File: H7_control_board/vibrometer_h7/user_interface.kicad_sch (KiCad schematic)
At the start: 21 parts, among them J501 Conn_02x12_Counter_Clockwise, SW501 SW_Push, SW502 SW_Push

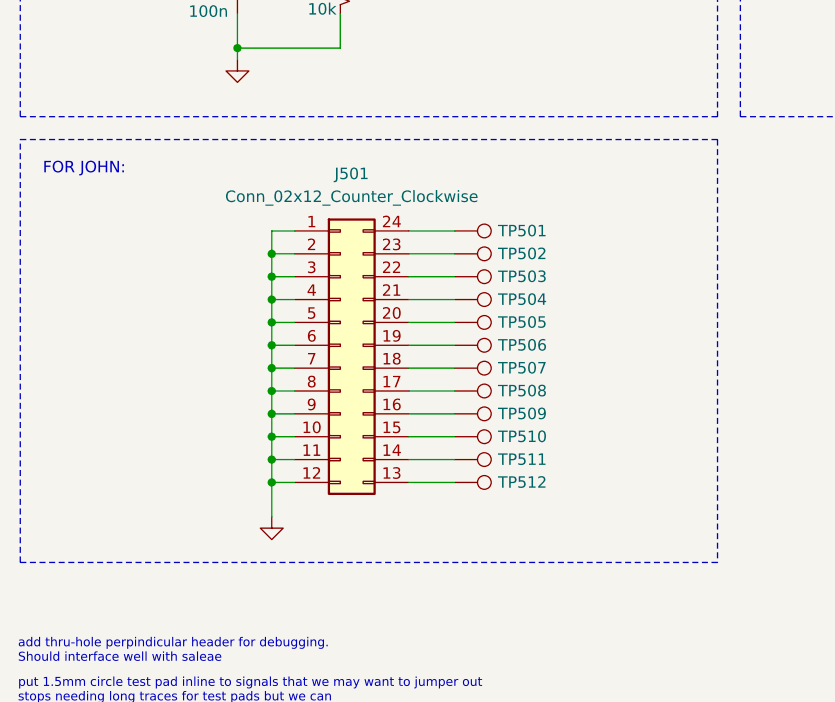
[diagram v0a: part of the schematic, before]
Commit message: lots of routing progress!!
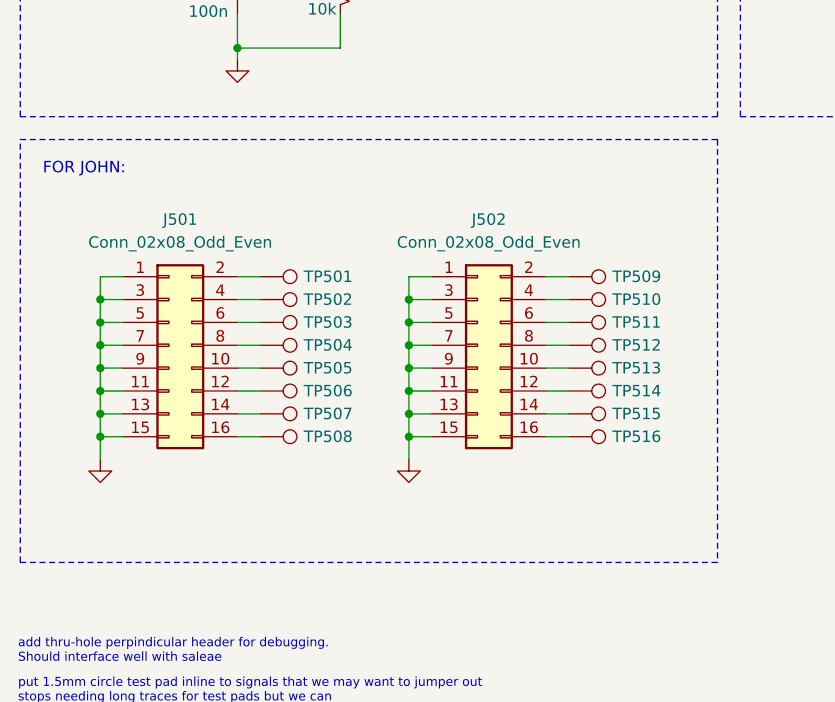
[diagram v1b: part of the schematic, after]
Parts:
- removed J501: Conn_02x12_Counter_Clockwise, symbol Connector_Generic:Conn_02x12_Counter_Clockwise
- added J501, J502: Conn_02x08_Odd_Even, Connector_PinHeader_1.00mm:PinHeader_2x08_P1.00mm_Vertical_SMD, symbol Connector_Generic:Conn_02x08_Odd_Even
- added TP513, TP514, TP515, TP516: TestPoint, TestPoint:TestPoint_Pad_D1.0mm, symbol Connector:TestPoint
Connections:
- net GND: now also J501.1 (Pin_1), J501.11 (Pin_11), J501.13 (Pin_13), J501.15 (Pin_15), J501.3 (Pin_3), J501.5 (Pin_5), J501.7 (Pin_7), J501.9 (Pin_9), J502.1 (Pin_1), J502.11 (Pin_11), J502.13 (Pin_13), J502.15 (Pin_15), J502.3 (Pin_3), J502.5 (Pin_5), J502.7 (Pin_7), J502.9 (Pin_9)
- net at TP512.1: now also J502.8 (Pin_8)
- net at TP504.1: now also J501.8 (Pin_8)
- net at TP507.1: now also J501.14 (Pin_14)
- net at TP511.1: now also J502.6 (Pin_6)
- net at TP510.1: now also J502.4 (Pin_4)
- net at TP509.1: now also J502.2 (Pin_2)
- net at TP508.1: now also J501.16 (Pin_16)
- net at TP506.1: now also J501.12 (Pin_12)
- net at TP505.1: now also J501.10 (Pin_10)
- net at TP503.1: now also J501.6 (Pin_6)
- net at TP502.1: now also J501.4 (Pin_4)
- net at TP501.1: now also J501.2 (Pin_2)
- new net: J502.12 (Pin_12), TP514.1
- new net: J502.16 (Pin_16), TP516.1
- new net: J502.14 (Pin_14), TP515.1
- new net: J502.10 (Pin_10), TP513.1
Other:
- moved on the sheet: TP501, TP502, TP503, TP504, TP505, TP506, TP507, TP508
